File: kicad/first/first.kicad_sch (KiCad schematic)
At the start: 2 parts, among them U1 PN532_Board, U2 WeMos_D1_mini

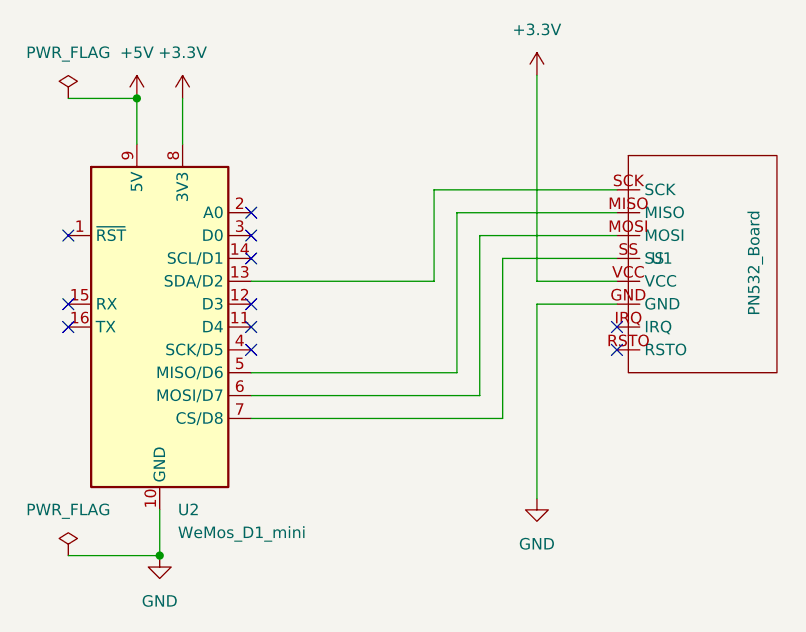
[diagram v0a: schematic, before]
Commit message: update kicad/first
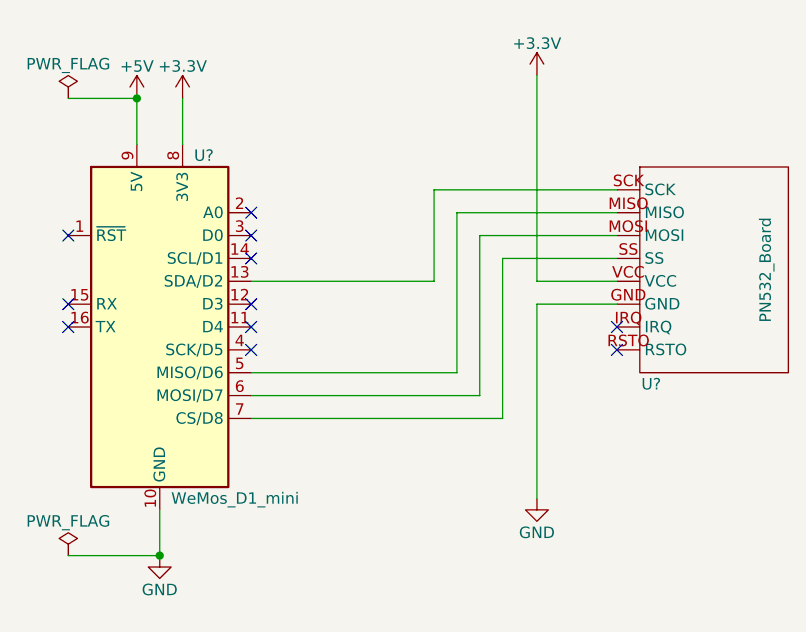
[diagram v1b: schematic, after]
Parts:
- renumbered U2 to U?, U1 to U?
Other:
- moved on the sheet: U?
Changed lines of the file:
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@@
   (symbol (lib_id "power:GND") (at 96.52 128.27 0) (unit 1)
     (in_bom yes) (on_board yes) (fields_autoplaced)
-    (property "Reference" "#PWR0104" (id 0) (at 96.52 134.62 0)
+    (property "Reference" "#PWR?" (id 0) (at 96.52 134.62 0)
       (effects (font (size 1.27 1.27)) hide)
     )
-    (property "Value" "GND" (id 1) (at 96.52 133.35 0))
+    (property "Value" "GND" (id 1) (at 96.52 132.08 0))
     (property "Footprint" "" (id 2) (at 96.52 128.27 0)
       (effects (font (size 1.27 1.27)) hide)
@@
   (symbol (lib_id "power:PWR_FLAG") (at 44.45 134.62 0) (unit 1)
     (in_bom yes) (on_board yes) (fields_autoplaced)
-    (property "Reference" "#FLG0101" (id 0) (at 44.45 132.715 0)
+    (property "Reference" "#FLG?" (id 0) (at 44.45 132.715 0)
       (effects (font (size 1.27 1.27)) hide)
     )
-    (property "Value" "PWR_FLAG" (id 1) (at 44.45 129.54 0))
+    (property "Value" "PWR_FLAG" (id 1) (at 44.45 130.81 0))
     (property "Footprint" "" (id 2) (at 44.45 134.62 0)
       (effects (font (size 1.27 1.27)) hide)
@@
   (symbol (lib_id "power:+3.3V") (at 96.52 81.28 0) (unit 1)
     (in_bom yes) (on_board yes) (fields_autoplaced)
-    (property "Reference" "#PWR0105" (id 0) (at 96.52 85.09 0)
+    (property "Reference" "#PWR?" (id 0) (at 96.52 85.09 0)
       (effects (font (size 1.27 1.27)) hide)
     )
-    (property "Value" "+3.3V" (id 1) (at 96.52 76.2 0))
+    (property "Value" "+3.3V" (id 1) (at 96.52 77.724 0))
     (property "Footprint" "" (id 2) (at 96.52 81.28 0)
       (effects (font (size 1.27 1.27)) hide)
@@
   (symbol (lib_id "power:+5V") (at 52.07 83.82 0) (unit 1)
     (in_bom yes) (on_board yes)
-    (property "Reference" "#PWR0102" (id 0) (at 52.07 87.63 0)
+    (property "Reference" "#PWR?" (id 0) (at 52.07 87.63 0)
       (effects (font (size 1.27 1.27)) hide)
     )
-    (property "Value" "+5V" (id 1) (at 52.07 78.74 0))
+    (property "Value" "+5V" (id 1) (at 52.07 80.264 0))
     (property "Footprint" "" (id 2) (at 52.07 83.82 0)
       (effects (font (size 1.27 1.27)) hide)
@@
   (symbol (lib_id "power:GND") (at 54.61 134.62 0) (unit 1)
     (in_bom yes) (on_board yes) (fields_autoplaced)
-    (property "Reference" "#PWR0101" (id 0) (at 54.61 140.97 0)
+    (property "Reference" "#PWR?" (id 0) (at 54.61 140.97 0)
       (effects (font (size 1.27 1.27)) hide)
     )
-    (property "Value" "GND" (id 1) (at 54.61 139.7 0))
+    (property "Value" "GND" (id 1) (at 54.61 138.43 0))
     (property "Footprint" "" (id 2) (at 54.61 134.62 0)
       (effects (font (size 1.27 1.27)) hide)
@@
   (symbol (lib_id "power:+3.3V") (at 57.15 83.82 0) (unit 1)
     (in_bom yes) (on_board yes) (fields_autoplaced)
-    (property "Reference" "#PWR0103" (id 0) (at 57.15 87.63 0)
+    (property "Reference" "#PWR?" (id 0) (at 57.15 87.63 0)
       (effects (font (size 1.27 1.27)) hide)
     )
-    (property "Value" "+3.3V" (id 1) (at 57.15 78.74 0))
+    (property "Value" "+3.3V" (id 1) (at 57.15 80.264 0))
     (property "Footprint" "" (id 2) (at 57.15 83.82 0)
       (effects (font (size 1.27 1.27)) hide)
@@
   (symbol (lib_id "MCU_Module:WeMos_D1_mini") (at 54.61 109.22 0) (unit 1)
     (in_bom yes) (on_board yes) (fields_autoplaced)
-    (property "Reference" "U2" (id 0) (at 56.6294 129.54 0)
+    (property "Reference" "U?" (id 0) (at 58.42 90.17 0)
       (effects (font (size 1.27 1.27)) (justify left))
     )
-    (property "Value" "WeMos_D1_mini" (id 1) (at 56.6294 132.08 0)
+    (property "Value" "WeMos_D1_mini" (id 1) (at 55.88 128.27 0)
       (effects (font (size 1.27 1.27)) (justify left))
     )
@@
     (pin "9")
   )
-  (symbol (lib_id "New_Library:PN532_Board") (at 105.41 100.33 0) (unit 1)
+  (symbol (lib_id "New_Library:PN532_Board") (at 116.84 102.87 0) (unit 1)
     (in_bom yes) (on_board yes)
-    (property "Reference" "U1" (id 0) (at 109.22 101.5999 0)
-      (effects (font (size 1.27 1.27)) (justify left))
-    )
-    (property "Value" "PN532_Board" (id 1) (at 120.65 107.95 90)
-      (effects (font (size 1.27 1.27)) (justify left))
-    )
-    (property "Footprint" "Library:PN532_Board" (id 2) (at 105.41 100.33 0)
+    (property "Reference" "U?" (id 0) (at 109.22 115.57 0))
+    (property "Value" "PN532_Board" (id 1) (at 121.92 102.87 90))
+    (property "Footprint" "Library:PN532_Board" (id 2) (at 116.84 102.87 0)
       (effects (font (size 1.27 1.27)) hide)
     )
-    (property "Datasheet" "" (id 3) (at 105.41 100.33 0)
+    (property "Datasheet" "" (id 3) (at 116.84 102.87 0)
       (effects (font (size 1.27 1.27)) hide)
     )
@@
   (symbol (lib_id "power:PWR_FLAG") (at 44.45 83.82 0) (unit 1)
     (in_bom yes) (on_board yes) (fields_autoplaced)
-    (property "Reference" "#FLG0102" (id 0) (at 44.45 81.915 0)
+    (property "Reference" "#FLG?" (id 0) (at 44.45 81.915 0)
       (effects (font (size 1.27 1.27)) hide)
     )
-    (property "Value" "PWR_FLAG" (id 1) (at 44.45 78.74 0))
+    (property "Value" "PWR_FLAG" (id 1) (at 44.45 80.01 0))
     (property "Footprint" "" (id 2) (at 44.45 83.82 0)
       (effects (font (size 1.27 1.27)) hide)
@@
   (symbol_instances
     (path "/38123ca9-7ebf-4a0b-a442-cd99727995f5"
-      (reference "#FLG0101") (unit 1) (value "PWR_FLAG") (footprint "")
+      (reference "#FLG?") (unit 1) (value "PWR_FLAG") (footprint "")
     )
     (path "/fb051e16-8a37-43d3-9918-54d7e755e61c"
-      (reference "#FLG0102") (unit 1) (value "PWR_FLAG") (footprint "")
+      (reference "#FLG?") (unit 1) (value "PWR_FLAG") (footprint "")
+    )
+    (path "/27f75db7-cd04-4a08-90e5-250b77d098fd"
+      (reference "#PWR?") (unit 1) (value "GND") (footprint "")
+    )
+    (path "/46e66528-adaf-45db-86ff-2d0da7850450"
+      (reference "#PWR?") (unit 1) (value "+3.3V") (footprint "")
+    )
+    (path "/5a4d838c-8c38-4897-9a17-3071313b6654"
+      (reference "#PWR?") (unit 1) (value "+5V") (footprint "")
     )
     (path "/62f9483e-d02e-4474-9007-a01a7db7062a"
-      (reference "#PWR0101") (unit 1) (value "GND") (footprint "")
-    )
-    (path "/5a4d838c-8c38-4897-9a17-3071313b6654"
-      (reference "#PWR0102") (unit 1) (value "+5V") (footprint "")
+      (reference "#PWR?") (unit 1) (value "GND") (footprint "")
     )
     (path "/960ec519-144d-43cd-8c7d-4dd117f65b95"
-      (reference "#PWR0103") (unit 1) (value "+3.3V") (footprint "")
+      (reference "#PWR?") (unit 1) (value "+3.3V") (footprint "")
     )
-    (path "/27f75db7-cd04-4a08-90e5-250b77d098fd"
-      (reference "#PWR0104") (unit 1) (value "GND") (footprint "")
-    )
-    (path "/46e66528-adaf-45db-86ff-2d0da7850450"
-      (reference "#PWR0105") (unit 1) (value "+3.3V") (footprint "")
+    (path "/a76a03cf-64af-44c7-be09-ddff38e2abe9"
+      (reference "U?") (unit 1) (value "WeMos_D1_mini") (footprint "Module:WEMOS_D1_mini_light")
     )
     (path "/f894cbb8-b9d5-440f-aa02-3b99f1bbb01a"
-      (reference "U1") (unit 1) (value "PN532_Board") (footprint "Library:PN532_Board")
-    )
-    (path "/a76a03cf-64af-44c7-be09-ddff38e2abe9"
-      (reference "U2") (unit 1) (value "WeMos_D1_mini") (footprint "Module:WEMOS_D1_mini_light")
+      (reference "U?") (unit 1) (value "PN532_Board") (footprint "Library:PN532_Board")
     )
   )
